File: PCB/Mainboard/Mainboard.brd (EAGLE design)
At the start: 39.1 x 39.1 mm, 18 parts

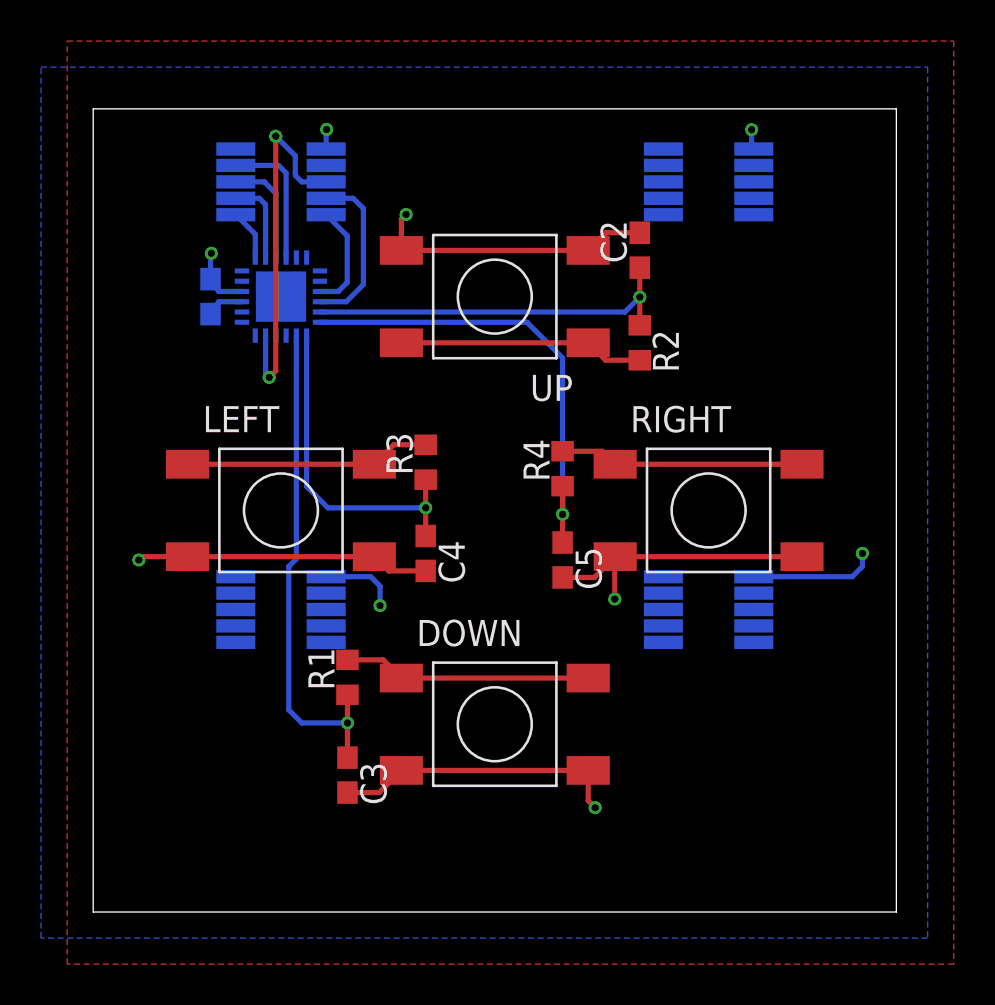
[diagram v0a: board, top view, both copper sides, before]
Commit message: Redesign
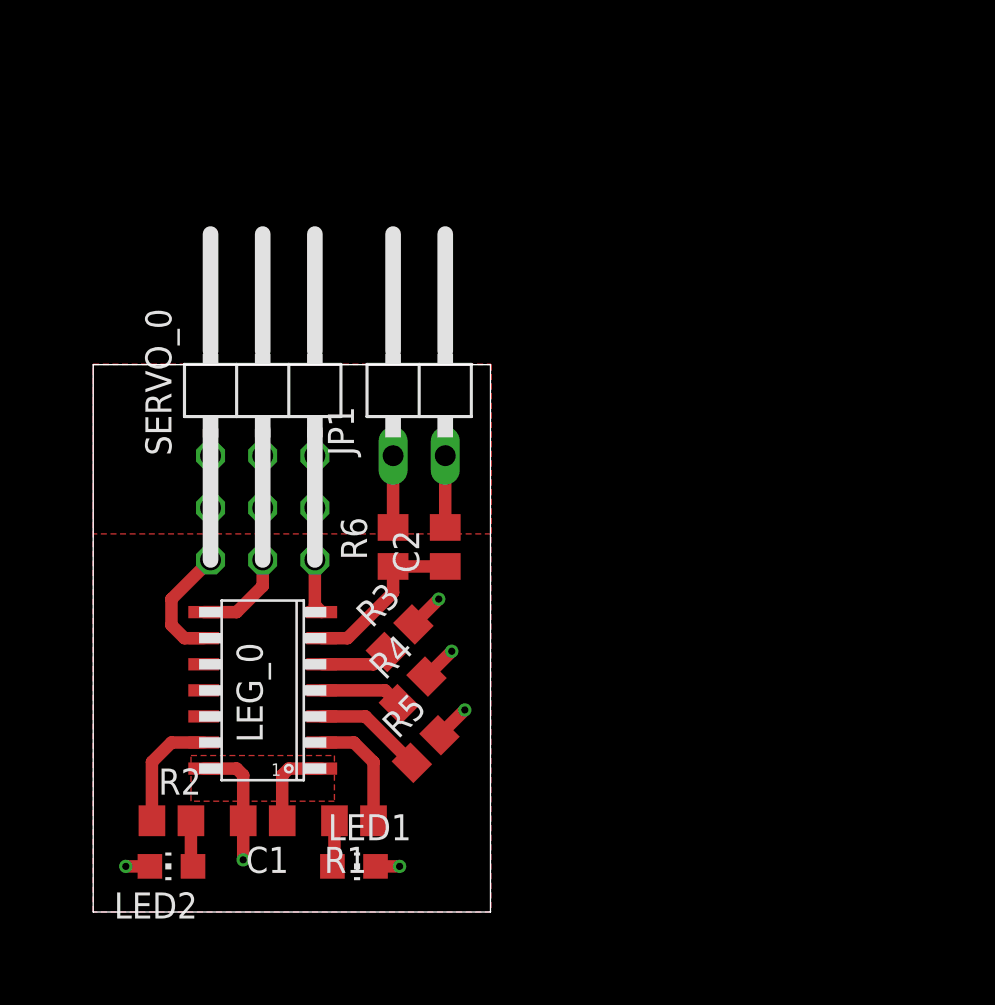
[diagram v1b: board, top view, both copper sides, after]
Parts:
- removed C3, C4, C5: 20nF, rcl:C0603
- removed DOWN, LEFT, RIGHT, UP: TASTER, button:TASTER
- removed MCU: ATTINY1614/16/17, ATTINY161x:QFN24-4X4
- removed U$1, U$2, U$3, U$4: MOLEX-STACKINGHEADER, Molex-53307-1071:53307-1071
- added JP1: (no value), pinhead:1X02/90
- added LED1, LED2: (no value), led:CHIP-LED0805
- added LEG_0: ATTINY1614, HeRo:SOIC14
- added R5, R6: (no value), rcl:R0805
- added SERVO_0: SERVO_X3, HeRo:2X03/90
- C1: value 100nF -> (none); device rcl:C0603 -> rcl:C0805
- C2: value 20nF -> (none); device rcl:C0603 -> rcl:C0805
- R1, R2, R3, R4: value 1k -> (none); device rcl:R0603 -> rcl:R0805
- moved R2 32.6 mm to (3.81, 4.45), turned to 0 degrees
- moved C1 25.7 mm to (8.26, 4.45), flipped to the top, turned to 180 degrees
- moved C2 17.3 mm to (17.1, 17.8)
- moved R4 13.0 mm to (15.6, 10.8), turned to 45 degrees
- moved R3 8.67 mm to (14.9, 13.3), turned to 45 degrees
- moved R1 6.99 mm to (12.7, 4.45), turned to 180 degrees
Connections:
- removed net ADD0: MCU.7, U$1.P$6
- removed net ADD1: MCU.8, U$1.P$7
- removed net ADD2: MCU.9, U$1.P$8
- removed net ADD3: MCU.10, U$1.P$9
- removed net DOWN: C3.1, MCU.20, R1.1
- removed net LEFT: C4.1, MCU.19, R3.1
- removed net N$3: R2.2, UP.A0, UP.A1
- removed net RIGHT: C5.1, MCU.18, R4.1
- removed net UP: C2.1, MCU.17, R2.1
- removed net UPDI: MCU.23, U$1.P$3
- new net ADDA_0: LEG_0.5, R3.1
- new net ADDB_0: LEG_0.4, R4.1
- new net ADDC_0: LEG_0.3, R5.1
- new net LEDA_0: LEG_0.2, R1.1
- new net LEDB_0: LEG_0.13, R2.1
- new net PWMA_0: LEG_0.9, SERVO_0.1
- new net PWMB_0: LEG_0.8, SERVO_0.2
- new net PWMC_0: LEG_0.7, SERVO_0.3
- new net SENSE_0: C2.1, LEG_0.6, R6.1
- new net UPDI_0: LEG_0.10
- new net VDD: SERVO_0.4, SERVO_0.5, SERVO_0.6
- net +5V: now also LEG_0.1; no longer MCU.4, U$1.P$1, U$2.P$1, U$3.P$1, U$4.P$1
- net GND: now also JP1.2, LED1.C, LED2.C, LEG_0.14, R3.2, R4.2, R5.2, SERVO_0.7, SERVO_0.8, SERVO_0.9; no longer C3.2, C4.2, C5.2, DOWN.B0, DOWN.B1, LEFT.B0, LEFT.B1, MCU.3, RIGHT.B0, RIGHT.B1, U$1.P$10, U$2.P$10, U$3.P$10, U$4.P$10, UP.B0, UP.B1
- net N$1: now also LED1.A; no longer DOWN.A0, DOWN.A1
- net N$2: now also LED2.A, R2.2; no longer LEFT.A0, LEFT.A1, R3.2
- net N$4: now also JP1.1, R6.2; no longer R4.2, RIGHT.A0, RIGHT.A1
- net SCL: now also LEG_0.12; no longer MCU.16, U$1.P$4
- net SDA: now also LEG_0.11; no longer MCU.15, U$1.P$5
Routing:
- net GND: track 58.3 -> 17.3 mm, vias 4 -> 6
- net DOWN: track 24.6 -> 0.00 mm, vias 1 -> 0
- net RIGHT: track 22.9 -> 0.00 mm, vias 1 -> 0
- net UP: track 18.7 -> 0.00 mm, vias 1 -> 0
- net UPDI: track 17.9 -> 0.00 mm, vias 2 -> 0
- net LEFT: track 16.3 -> 0.00 mm, vias 1 -> 0
- net N$3: track 12.0 -> 0.00 mm
- net +5V: track 15.0 -> 4.28 mm, vias 5 -> 0
- net N$1: track 12.1 -> 2.26 mm
- net N$2: track 12.0 -> 2.26 mm
- net N$4: track 11.9 -> 3.50 mm
- net SENSE_0: track 0.00 -> 8.21 mm
- net SCL: track 8.19 -> 0.00 mm
- net ADD3: track 6.72 -> 0.00 mm
- net PWMA_0: track 0.00 -> 5.80 mm
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- added copper zone on layer 1, net N$3
- added copper zone on layer 1, net VDD
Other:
- board size 39.1 x 39.1 mm -> 19.3 x 26.7 mm
